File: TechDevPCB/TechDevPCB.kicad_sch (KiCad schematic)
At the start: 15 parts, among them J1 Screw_Terminal_01x02, J10 Conn_01x05_Pin, J2 Screw_Terminal_01x02, J3 Conn_01x02_Pin, J4 Conn_01x04_Pin, J5 Conn_01x02_Pin, J6 Conn_01x04_Pin, J8 Conn_01x05_Pin, J9 Conn_01x05_Pin, U1 DRV8825_STEPPER_MOTOR_DRIVER_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, U2 DRV8825_STEPPER_MOTOR_DRIVER_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, U3 XL6009 Boost Converter

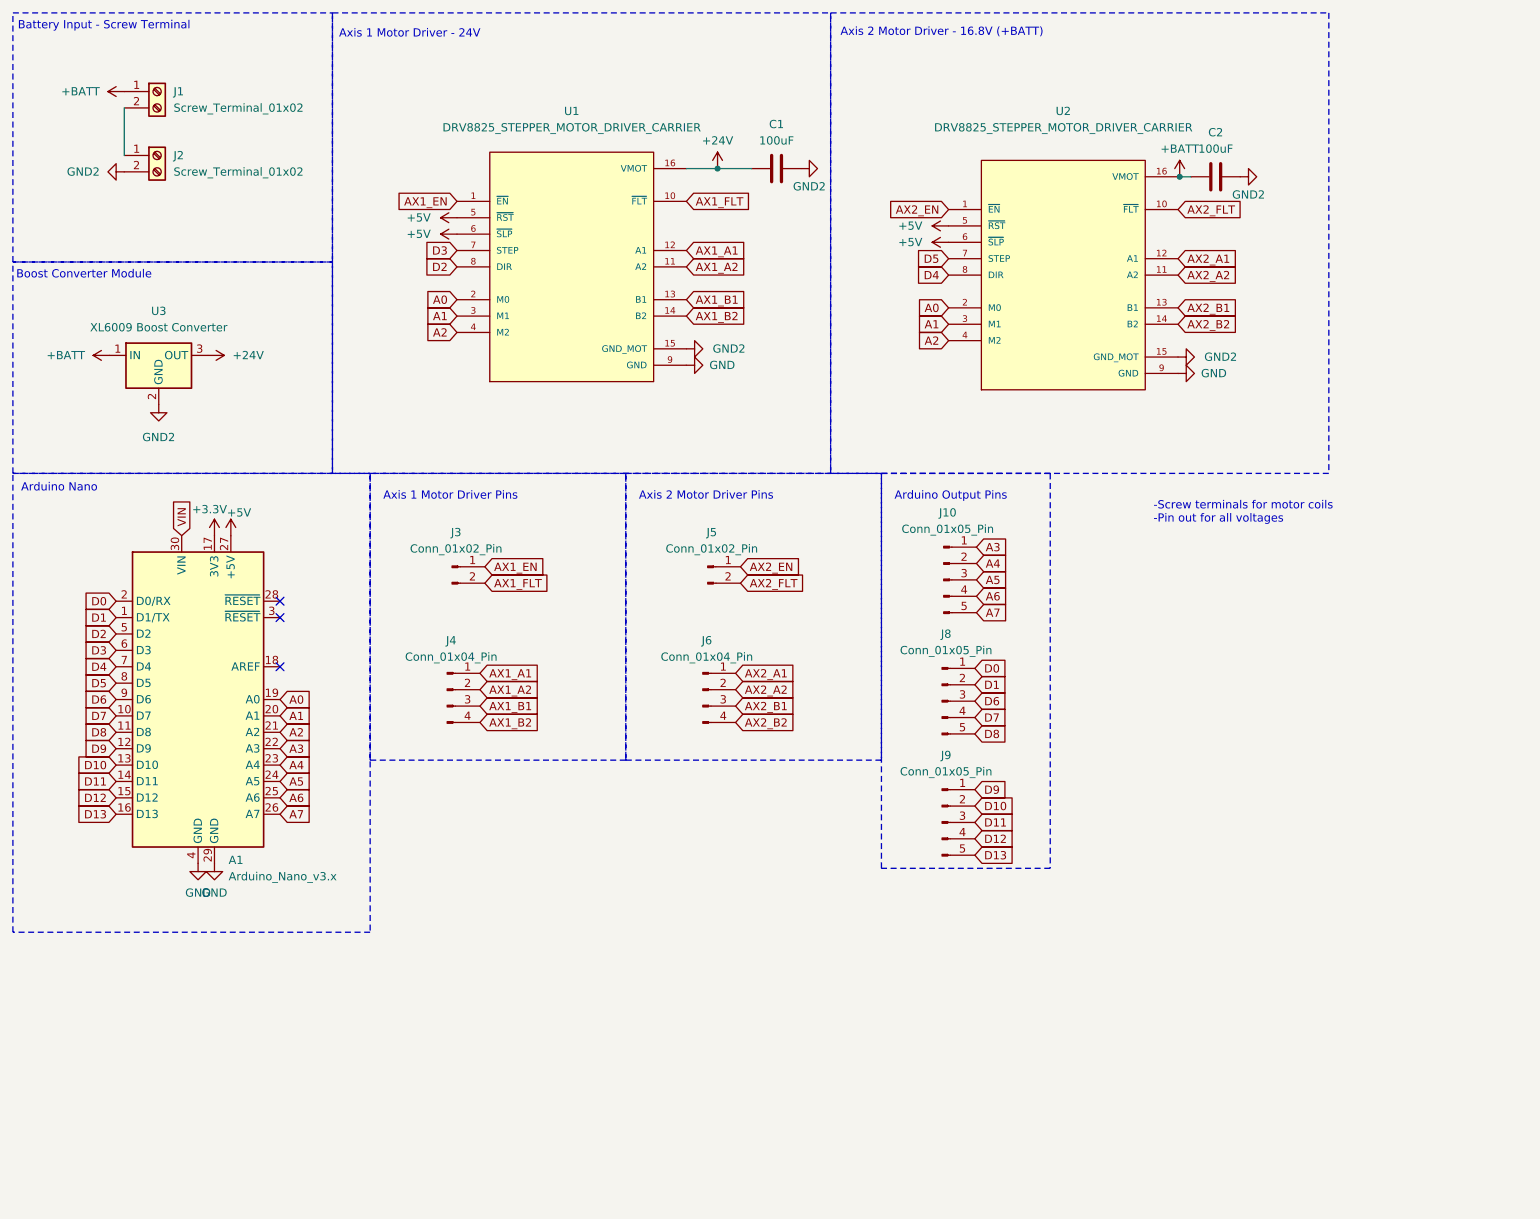
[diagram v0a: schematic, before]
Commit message: PCB Updates
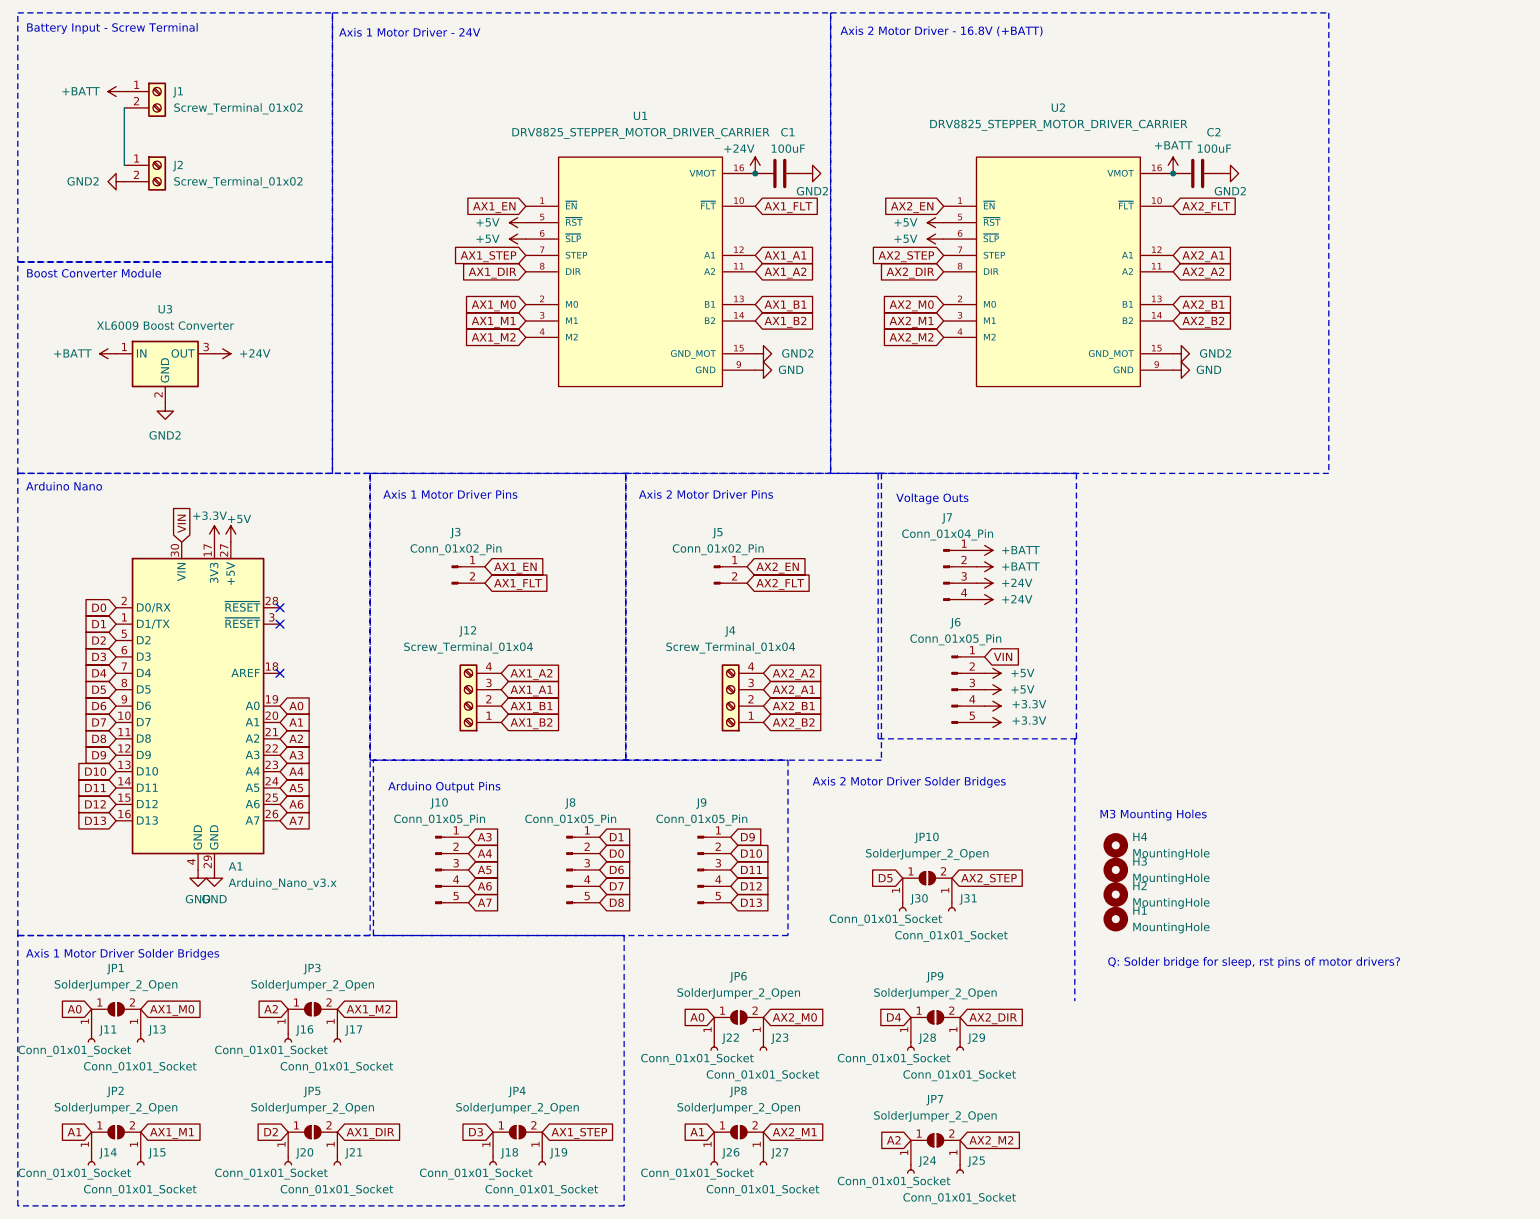
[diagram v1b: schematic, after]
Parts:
- removed J4, J6: Conn_01x04_Pin, Connector_PinHeader_2.54mm:PinHeader_1x04_P2.54mm_Vertical, symbol Connector:Conn_01x04_Pin
- added H1, H2, H3, H4: MountingHole, MountingHole:MountingHole_3.2mm_M3_DIN965, symbol Mechanical:MountingHole
- added J11, J13, J14, J15, J16, J17, J18, J19, J20, J21, J22, J23, J24, J25, J26, J27, J28, J29, J30, J31: Conn_01x01_Socket, Connector_PinHeader_2.54mm:PinHeader_1x01_P2.54mm_Vertical, symbol Connector:Conn_01x01_Socket
- added J12, J4: Screw_Terminal_01x04, TerminalBlock:TerminalBlock_bornier-4_P5.08mm, symbol Connector:Screw_Terminal_01x04
- added J6: Conn_01x05_Pin, Connector_PinHeader_2.54mm:PinHeader_1x05_P2.54mm_Vertical, symbol Connector:Conn_01x05_Pin
- added J7: Conn_01x04_Pin, Connector_PinHeader_2.54mm:PinHeader_1x04_P2.54mm_Vertical, symbol Connector:Conn_01x04_Pin
- added JP1, JP10, JP2, JP3, JP4, JP5, JP6, JP7, JP8, JP9: SolderJumper_2_Open, Jumper:SolderJumper-2_P1.3mm_Open_Pad1.0x1.5mm, symbol Jumper:SolderJumper_2_Open
- J2: footprint (none) -> TerminalBlock:TerminalBlock_bornier-2_P5.08mm
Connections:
- net +24V: now also J7.3 (Pin_3), J7.4 (Pin_4)
- net +3.3V: now also J6.4 (Pin_4), J6.5 (Pin_5)
- net +5V: now also J6.2 (Pin_2), J6.3 (Pin_3)
- net +BATT: now also J7.1 (Pin_1), J7.2 (Pin_2)
- net A0: now also J11.1 (Pin_1), J22.1 (Pin_1), JP1.1 (A), JP6.1 (A); no longer U1.2 (M0), U2.2 (M0)
- net A1: now also J14.1 (Pin_1), J26.1 (Pin_1), JP2.1 (A), JP8.1 (A); no longer U1.3 (M1), U2.3 (M1)
- net A2: now also J16.1 (Pin_1), J24.1 (Pin_1), JP3.1 (A), JP7.1 (A); no longer U1.4 (M2), U2.4 (M2)
- net AX1_A1: now also J12.3 (Pin_3)
- net AX1_A2: now also J12.4 (Pin_4)
- net AX1_B1: now also J12.2 (Pin_2)
- net AX1_B2: now also J12.1 (Pin_1)
- net AX2_A1: now also J4.3 (Pin_3)
- net AX2_A2: now also J4.4 (Pin_4)
- net AX2_B1: now also J4.2 (Pin_2)
- net AX2_B2: now also J4.1 (Pin_1)
- net D0: now also J8.2 (Pin_2); no longer J8.1 (Pin_1)
- net D1: now also J8.1 (Pin_1); no longer J8.2 (Pin_2)
- net D2: now also J20.1 (Pin_1), JP5.1 (A); no longer U1.8 (DIR)
- net D3: now also J18.1 (Pin_1), JP4.1 (A); no longer U1.7 (STEP)
- net D4: now also J28.1 (Pin_1), JP9.1 (A); no longer U2.8 (DIR)
- net D5: now also J30.1 (Pin_1), JP10.1 (A); no longer U2.7 (STEP)
- net VIN: now also J6.1 (Pin_1)
- new net AX1_DIR: J21.1 (Pin_1), JP5.2 (B), U1.8 (DIR)
- new net AX1_M0: J13.1 (Pin_1), JP1.2 (B), U1.2 (M0)
- new net AX1_M1: J15.1 (Pin_1), JP2.2 (B), U1.3 (M1)
- new net AX1_M2: J17.1 (Pin_1), JP3.2 (B), U1.4 (M2)
- new net AX1_STEP: J19.1 (Pin_1), JP4.2 (B), U1.7 (STEP)
- new net AX2_DIR: J29.1 (Pin_1), JP9.2 (B), U2.8 (DIR)
- new net AX2_M0: J23.1 (Pin_1), JP6.2 (B), U2.2 (M0)
- new net AX2_M1: J27.1 (Pin_1), JP8.2 (B), U2.3 (M1)
- new net AX2_M2: J25.1 (Pin_1), JP7.2 (B), U2.4 (M2)
- new net AX2_STEP: J31.1 (Pin_1), JP10.2 (B), U2.7 (STEP)
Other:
- note added: "Axis 1 Motor Driver Solder Bridges"
- note added: "Axis 2 Motor Driver Solder Bridges"
- note added: "M3 Mounting Holes"
- note added: "Q: Solder bridge for sleep, rst pins of motor drivers?"
- note added: "Voltage Outs"
- note removed: "-Screw terminals for motor coils -Pin out for all voltages"
- moved on the sheet: A1, C1, J2, J5, U1, U2, U3
